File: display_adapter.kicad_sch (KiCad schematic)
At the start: 60 parts, among them J4 54104-5031, Q1 BSS138, Q2 SI2301CDS-T1-E3, Q31 AO3401A, Q32 S8050, U2 RT9193-33GB

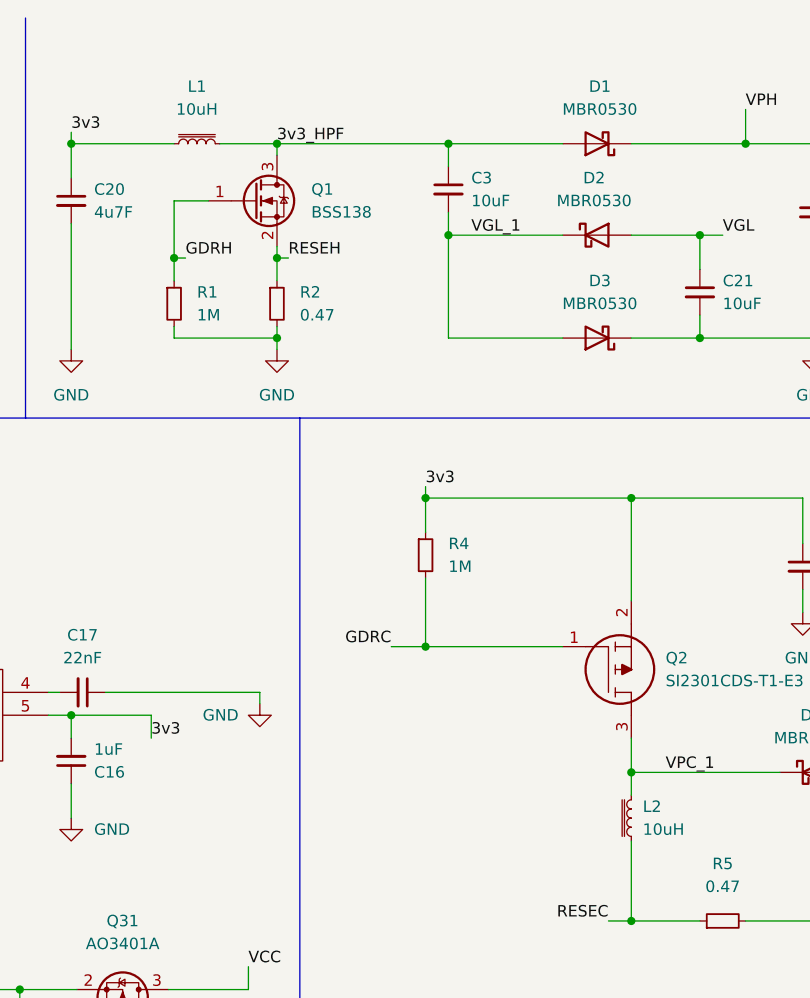
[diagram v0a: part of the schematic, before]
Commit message: Revision 1 of the board that was manufactured
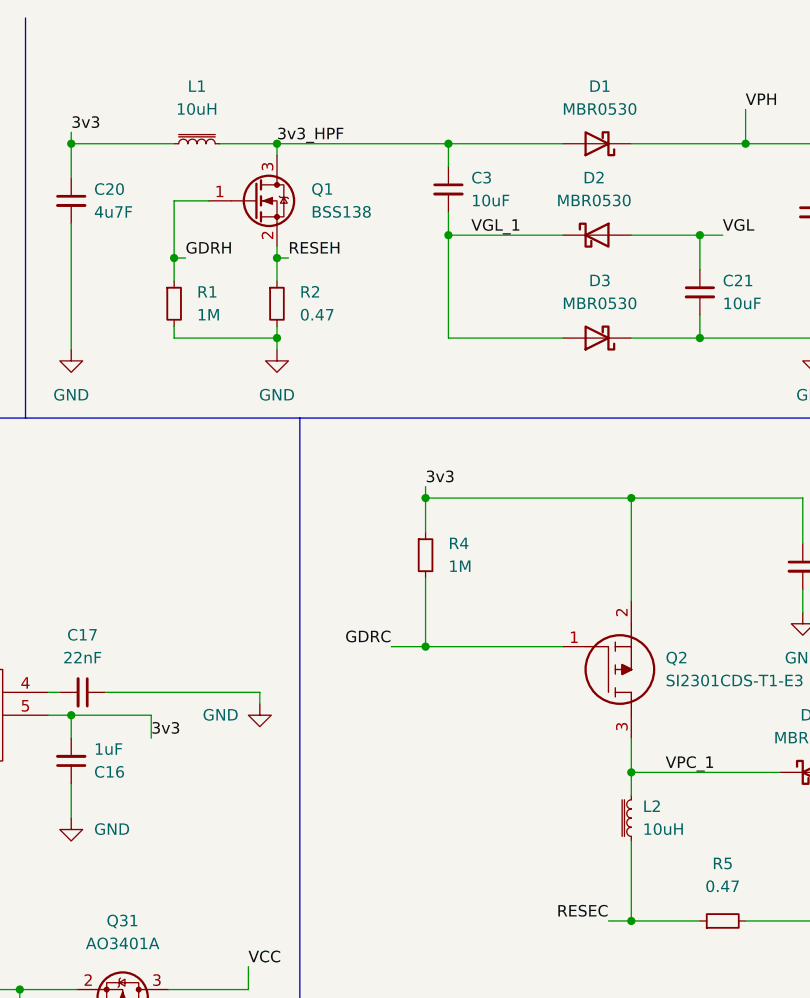
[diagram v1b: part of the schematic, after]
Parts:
- C1: LCSC (none) -> C19666; MAX Voltage (none) -> 10V; MAX voltage 10V -> (none)
- C10, C12, C21, C28, C3, C5, C6, C7, C8, C9: LCSC (none) -> C96446
- C11, C18, C24, C25, C26, C29: LCSC (none) -> C15849
- C14, C15: LCSC (none) -> C49678
- C16: LCSC (none) -> C28323
- C17: LCSC (none) -> C1729
- C19, C20: LCSC (none) -> C19666
- C2, C27: LCSC (none) -> C1623
- C23: LCSC (none) -> C23630
- C4: LCSC (none) -> C14663
- D1, D2, D3, D4: LCSC (none) -> C18863
- J4: LCSC (none) -> C505282
- L1, L2: LCSC (none) -> C82398
- Q1: LCSC (none) -> C82045
- Q2: LCSC (none) -> C145226
- Q31: LCSC (none) -> C15127
- Q32: footprint Package_TO_SOT_SMD:SOT-23 -> Package_TO_SOT_SMD:SOT-23-3; LCSC (none) -> C2150
- R1, R4: LCSC (none) -> C441966
- R2, R5: LCSC (none) -> C491238
- R27: LCSC (none) -> C149504
- R3, RA1, RB1: LCSC (none) -> C17477
- R33, R34: LCSC (none) -> C17713
- R35: LCSC (none) -> C510098
- R36: LCSC (none) -> C17513
- R37: LCSC (none) -> C2073899
- U2: LCSC (none) -> C15651
